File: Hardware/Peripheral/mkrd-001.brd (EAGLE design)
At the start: 18 x 31 mm, 5 parts

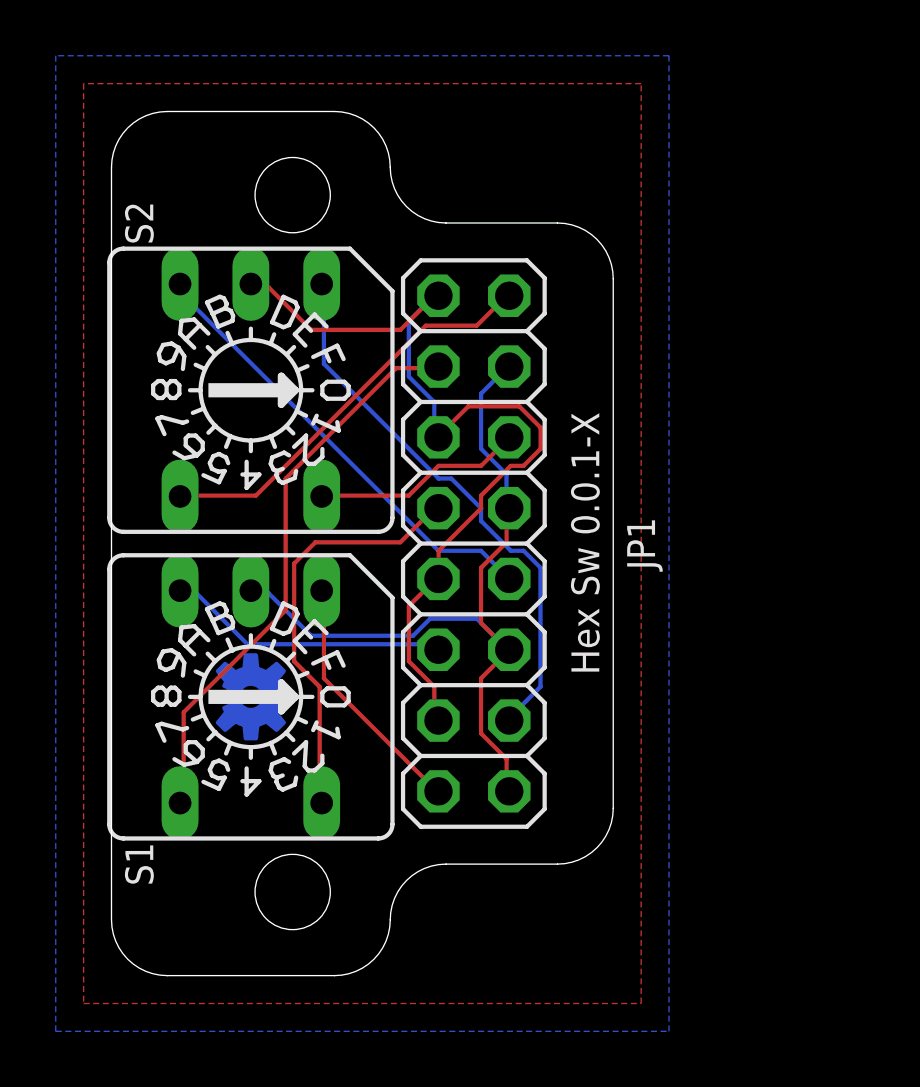
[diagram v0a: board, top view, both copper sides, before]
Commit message: First try.
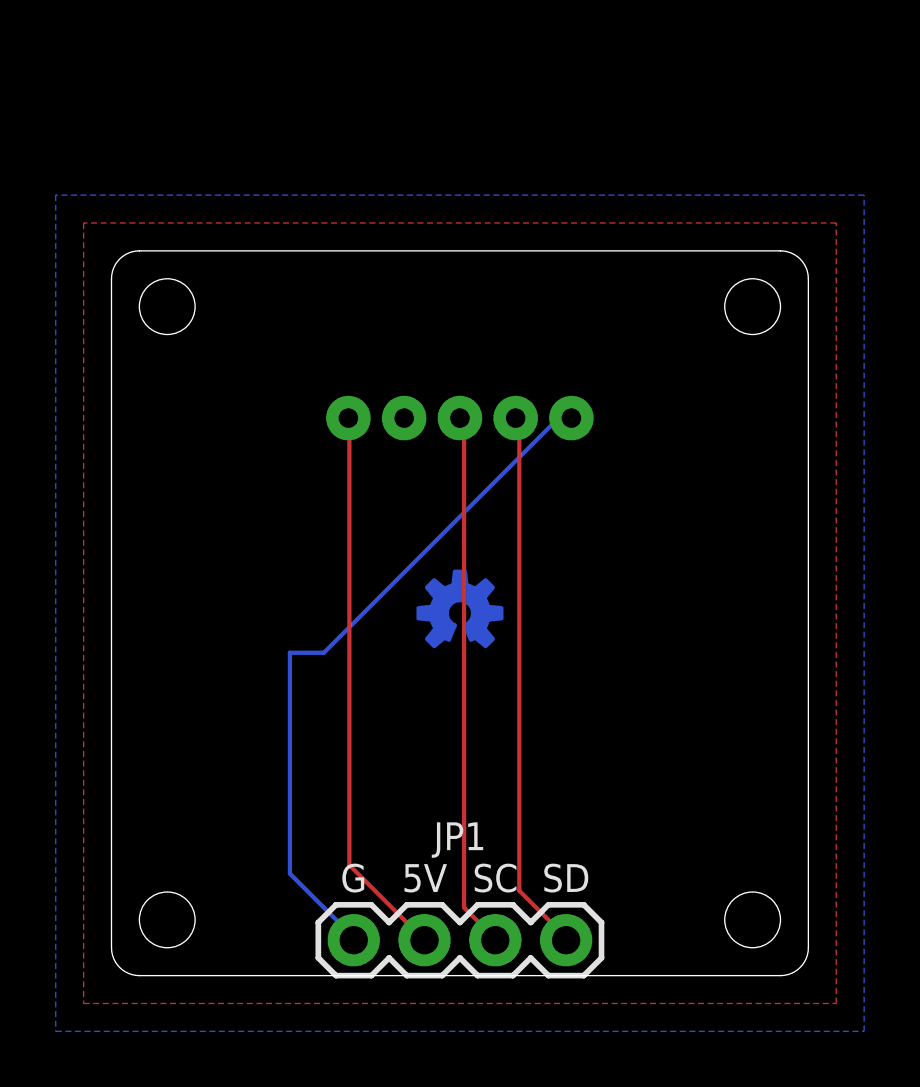
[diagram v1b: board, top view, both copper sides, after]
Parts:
- removed S1, S2: (no value), switch-dil:A1353HEX
- added J1: MKR, SparkFun-Connectors:JST-5-PTH
- JP1: value (none) -> DISP; device pinhead:2X08 -> SparkFun-Connectors:1X04
- moved U$1 18.4 mm to (12.5, 7.00), turned to 0 degrees
- moved JP1 14.9 mm to (8.69, 1.27), turned to 0 degrees
- moved LOGO1 8.08 mm to (12.5, 13.0), turned to 0 degrees
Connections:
- removed net ANLG0: JP1.3, S2.1
- removed net ANLG1: JP1.7, S2.4
- removed net ANLG2: JP1.11, S2.8
- removed net ANLG3: JP1.15, S2.2
- removed net DTCT0: JP1.2, S1.1
- removed net DTCT1: JP1.6, S1.4
- removed net DTCT2: JP1.10, S1.8
- removed net DTCT3: JP1.14, S1.2
- new net SCL: J1.3, JP1.3
- new net SDA: J1.2, JP1.4
- net GND: now also J1.1; no longer JP1.13, JP1.5, JP1.9, S1.C
- net VCC: now also J1.5, JP1.2; no longer JP1.12, JP1.16, JP1.4, JP1.8, S2.C
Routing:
- net DTCT3: track 20.4 -> 0.00 mm
- net ANLG0: track 19.9 -> 0.00 mm
- net SDA: track 0.00 -> 19.5 mm
- net SCL: track 0.00 -> 19.3 mm
- net ANLG1: track 16.4 -> 0.00 mm
- net DTCT2: track 15.0 -> 0.00 mm
- net ANLG3: track 14.8 -> 0.00 mm
- net VCC: track 31.7 -> 19.9 mm
- net DTCT1: track 10.1 -> 0.00 mm
- net DTCT0: track 8.95 -> 0.00 mm
- net ANLG2: track 7.60 -> 0.00 mm
- net GND: track 28.5 -> 24.8 mm
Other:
- board size 18 x 31 mm -> 25 x 26 mm
- board text added: "5V"
- board text added: "MKR Display 0.0.1-X"
- board text added: "SC"
- board text added: "SD"
- board text removed: "A0"
- board text removed: "A1"
- board text removed: "A2"
- board text removed: "A3"
- board text removed: "D10"
- board text removed: "D12"
- board text removed: "D6"
- board text removed: "D9"
- board text removed: "Hex Sw 0.0.1-X"
- board text removed: "V/2"
